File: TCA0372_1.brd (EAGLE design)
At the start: 100 x 80 mm, 30 parts, among them IC1R1 AQY212_1, IC2 Dil16: 4xAQY212, IC4 TCA0372, Q1 BSS101, Q2 BSS101

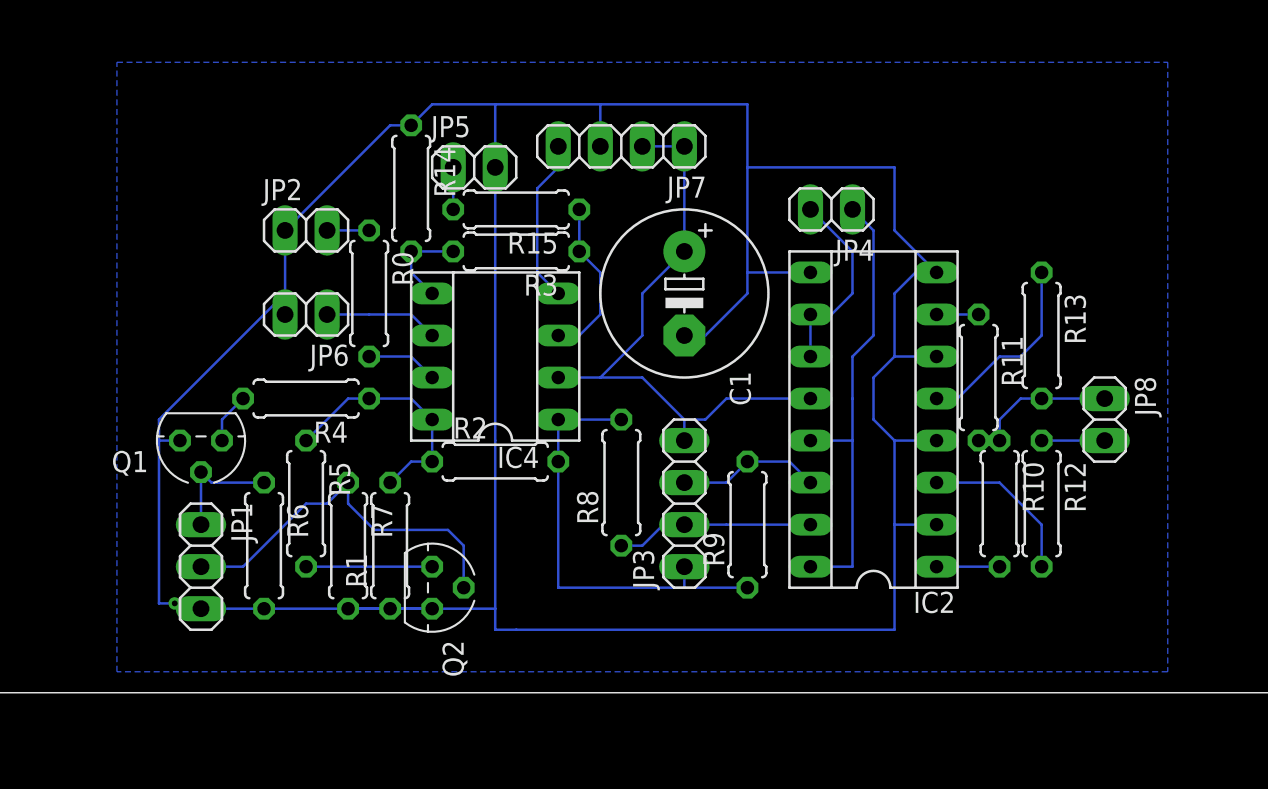
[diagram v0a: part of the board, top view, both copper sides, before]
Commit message: Add files via upload
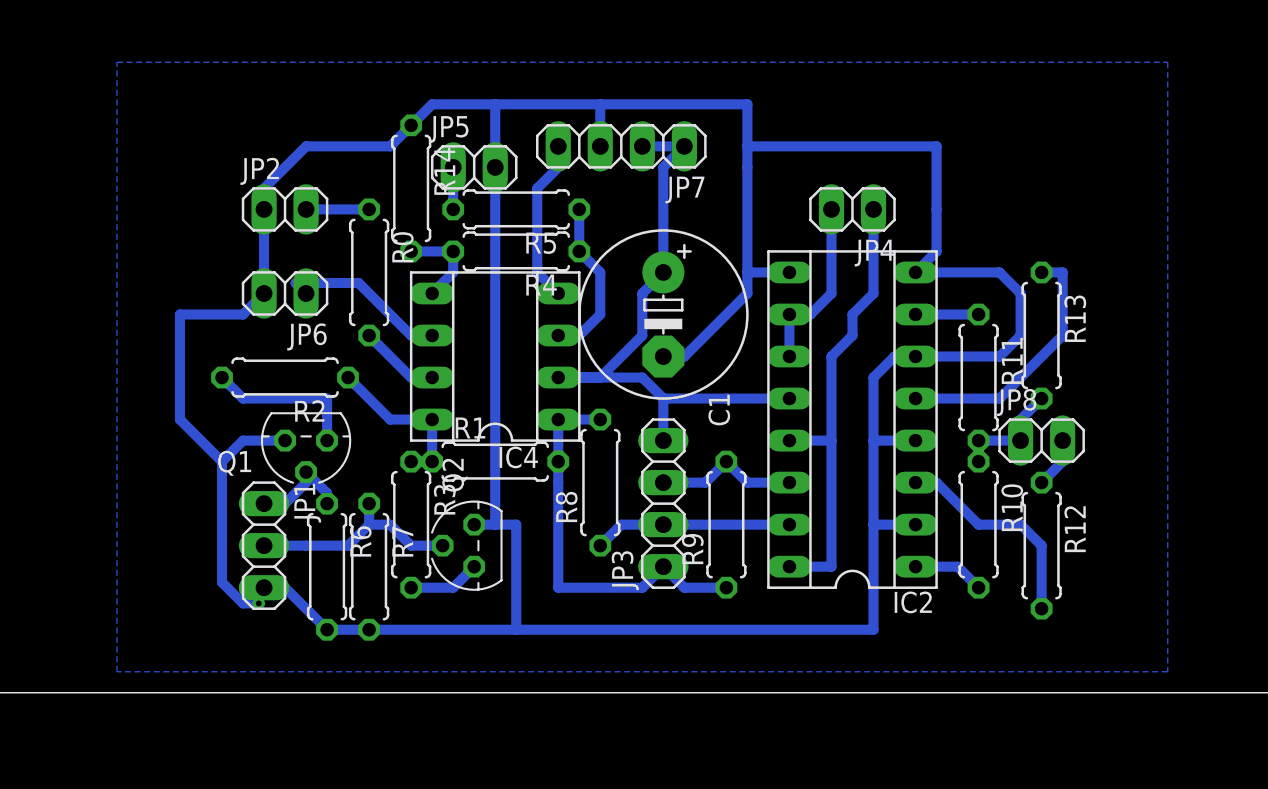
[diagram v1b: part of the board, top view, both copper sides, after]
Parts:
- removed R15: 27k, rcl:0207/7
- R14: value 33k -> 100M
- R3: value 68k -> 6.6k
- R4: value 33.2k -> 0
- R5: value 8.2k -> 0
- moved R5 21.8 mm to (39.4, 29.2), turned to 180 degrees
- moved R3 17.7 mm to (33.0, 10.2), turned to 270 degrees
- moved R4 15.5 mm to (39.4, 26.7)
- moved R2 13.7 mm to (25.4, 19.1), turned to 180 degrees
- moved R1 8.13 mm to (38.1, 14.0), turned to 0 degrees
- moved Q1 6.35 mm to (26.7, 15.2)
- moved JP8 4.02 mm to (71.1, 15.2), turned to 0 degrees
- moved R6 4.02 mm to (27.9, 7.62)
- moved JP1 4.02 mm to (24.1, 8.89)
- moved Q2 3.59 mm to (36.8, 8.89), turned to 90 degrees
- moved R12 2.54 mm to (71.1, 8.89)
- moved C1 1.80 mm to (48.3, 22.9)
- moved JP2 1.80 mm to (25.4, 29.2)
- moved JP6 1.80 mm to (25.4, 24.1)
- moved R7 1.80 mm to (30.5, 7.62)
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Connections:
- removed net N$14: IC4.1, JP3.1, R2.2, R8.2, R9.1
- removed net N$4: IC4.8, R1.2, R2.1, R4.1, R5.1
- new net N$21: IC4.1, JP3.1, R1.2, R8.2, R9.1
- new net N$22: IC4.8, R1.1, R2.1, R3.1
- net GND: no longer R1.1
- net N$1: now also R4.2; no longer R3.2
- net N$13: now also R4.1, R5.1; no longer R15.1, R3.1
- net N$20: now also R5.2; no longer R15.2
- net N$5: now also R2.2; no longer R4.2
- net N$6: now also R3.2; no longer R5.2
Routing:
- net N$14: track 26.7 -> 0.00 mm
- net N$21: track 0.00 -> 23.9 mm
- net N$4: track 14.8 -> 0.00 mm
- net N$22: track 0.00 -> 9.94 mm
- net N$8: track 22.8 -> 13.1 mm
- net N$5: track 3.07 -> 9.42 mm
- net GND: track 218.1 -> 223.5 mm
- net V+: track 36.7 -> 40.7 mm
- net N$15: track 11.7 -> 15.5 mm
- net N$9: track 6.88 -> 10.5 mm
- net N$6: track 7.62 -> 4.34 mm
- net N$10: track 9.94 -> 13.0 mm
- net N$19: track 9.42 -> 6.88 mm
- net N$12: track 2.54 -> 3.81 mm
- net N$18: track 2.54 -> 3.81 mm
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
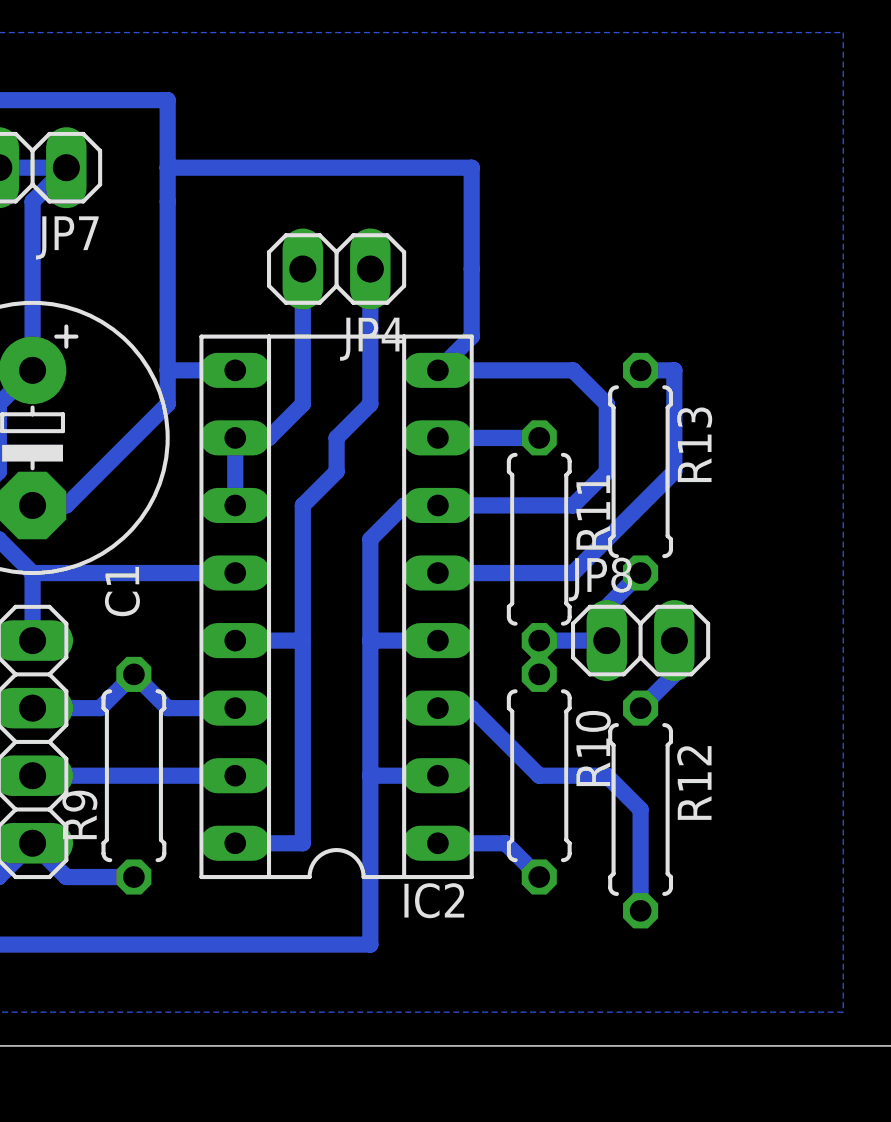
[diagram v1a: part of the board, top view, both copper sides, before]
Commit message: Add files via upload
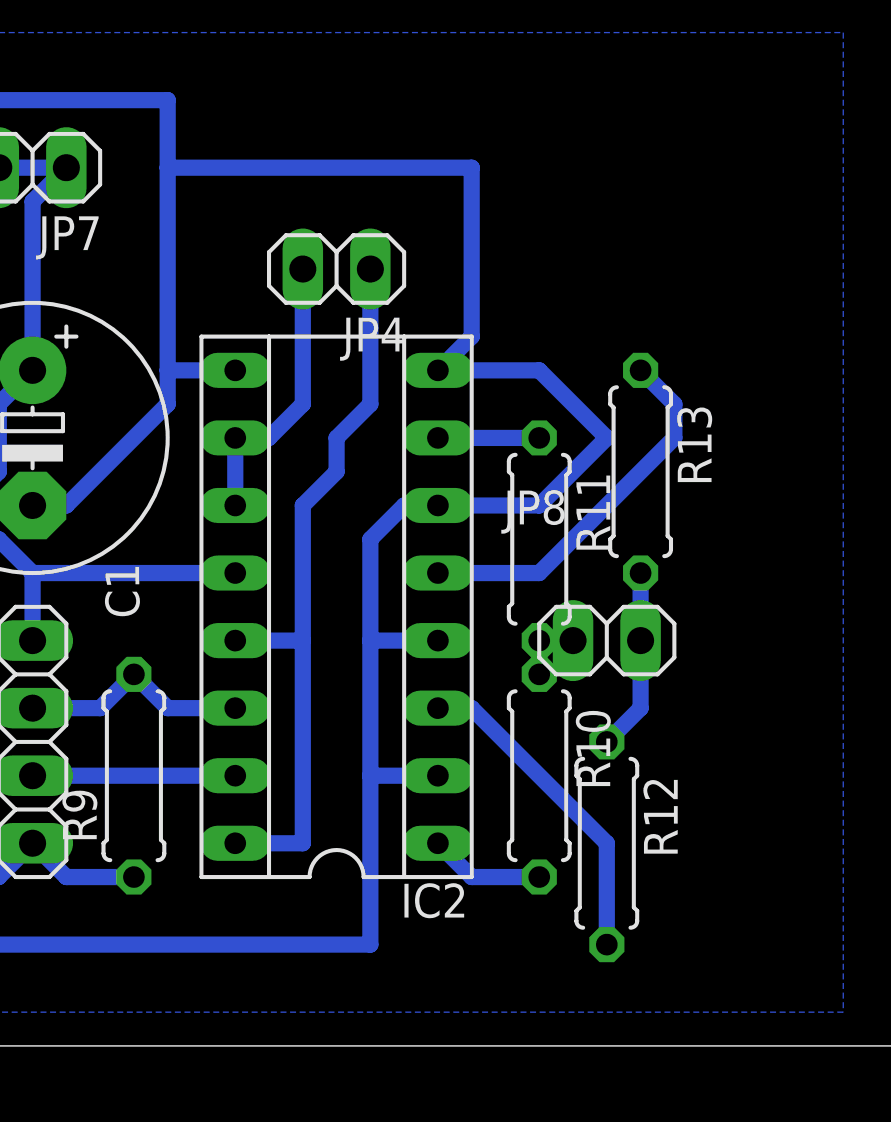
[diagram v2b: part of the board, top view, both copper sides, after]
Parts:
- JP8: value from Pin19/20 -> from Pin19->1/20->2
- moved R12 1.80 mm to (69.8, 7.62)
- moved JP8 1.27 mm to (69.8, 15.2)
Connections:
- net N$16: now also R13.2
- net N$19: no longer R13.2
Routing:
- net N$19: track 6.88 -> 2.54 mm
- net N$16: track 3.07 -> 6.88 mm
- net N$15: track 15.5 -> 14.1 mm
- net GND: track 223.5 -> 222.0 mm
- net N$10: track 13.0 -> 12.3 mm
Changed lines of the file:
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@@
 <attribute name="VALUE" x="62.23" y="32.385" size="1.27" layer="27" rot="R180"/>
 </element>
-<element name="JP8" library="pinhead" library_urn="urn:adsk.eagle:library:325" package="1X02" package3d_urn="urn:adsk.eagle:package:22435/2" value="from Pin19/20" x="71.12" y="15.24" smashed="yes">
-<attribute name="NAME" x="68.5038" y="17.0688" size="1.27" layer="25" ratio="10"/>
-<attribute name="VALUE" x="68.58" y="12.065" size="1.27" layer="27"/>
+<element name="JP8" library="pinhead" library_urn="urn:adsk.eagle:library:325" package="1X02" package3d_urn="urn:adsk.eagle:package:22435/2" value="from Pin19-&gt;1/20-&gt;2" x="69.85" y="15.24" smashed="yes">
+<attribute name="NAME" x="65.9638" y="19.6088" size="1.27" layer="25" ratio="10"/>
+<attribute name="VALUE" x="67.31" y="12.065" size="1.27" layer="27"/>
 </element>
 <element name="JP5" library="pinhead" library_urn="urn:adsk.eagle:library:325" package="1X02" package3d_urn="urn:adsk.eagle:package:22435/2" value="to Base" x="36.83" y="31.75" smashed="yes">
@@
 <attribute name="NAME" x="68.707" y="21.59" size="1.27" layer="25" ratio="10" rot="R270"/>
 <attribute name="SPICEPREFIX" value="R" x="67.31" y="19.05" size="1.778" layer="27" rot="R270" display="off"/>
-<attribute name="VALUE" x="66.7512" y="21.336" size="1.27" layer="27" ratio="10" rot="R270"/>
-</element>
-<element name="R12" library="rcl" library_urn="urn:adsk.eagle:library:334" package="0207/7" package3d_urn="urn:adsk.eagle:package:23493/1" value="470" x="71.12" y="8.89" smashed="yes" rot="R270">
-<attribute name="NAME" x="72.517" y="11.43" size="1.27" layer="25" ratio="10" rot="R270"/>
-<attribute name="SPICEPREFIX" value="R" x="71.12" y="8.89" size="1.778" layer="27" rot="R270" display="off"/>
-<attribute name="VALUE" x="70.5612" y="11.176" size="1.27" layer="27" ratio="10" rot="R270"/>
+<attribute name="VALUE" x="66.7512" y="20.066" size="1.27" layer="27" ratio="10" rot="R270"/>
+</element>
+<element name="R12" library="rcl" library_urn="urn:adsk.eagle:library:334" package="0207/7" package3d_urn="urn:adsk.eagle:package:23493/1" value="470" x="69.85" y="7.62" smashed="yes" rot="R270">
+<attribute name="NAME" x="71.247" y="10.16" size="1.27" layer="25" ratio="10" rot="R270"/>
+<attribute name="SPICEPREFIX" value="R" x="69.85" y="7.62" size="1.778" layer="27" rot="R270" display="off"/>
+<attribute name="VALUE" x="70.5612" y="9.906" size="1.27" layer="27" ratio="10" rot="R270"/>
 </element>
 <element name="R13" library="rcl" library_urn="urn:adsk.eagle:library:334" package="0207/7" package3d_urn="urn:adsk.eagle:package:23493/1" value="470" x="71.12" y="21.59" smashed="yes" rot="R270">
@@
 <wire x1="44.45" y1="35.56" x2="53.34" y2="35.56" width="0.6096" layer="16"/>
 <wire x1="53.34" y1="35.56" x2="53.34" y2="33.02" width="0.6096" layer="16"/>
-<wire x1="53.34" y1="31.75" x2="53.34" y2="25.4" width="0.6096" layer="16"/>
+<wire x1="53.34" y1="33.02" x2="53.34" y2="25.4" width="0.6096" layer="16"/>
 <wire x1="53.34" y1="25.4" x2="55.88" y2="25.4" width="0.6096" layer="16"/>
 <wire x1="48.26" y1="20.32" x2="49.53" y2="20.32" width="0.6096" layer="16"/>
@@
 <wire x1="36.83" y1="10.16" x2="38.1" y2="10.16" width="0.6096" layer="16"/>
 <wire x1="53.34" y1="33.02" x2="64.77" y2="33.02" width="0.6096" layer="16"/>
-<wire x1="64.77" y1="33.02" x2="64.77" y2="29.21" width="0.6096" layer="16"/>
-<wire x1="64.77" y1="29.21" x2="64.77" y2="26.67" width="0.6096" layer="16"/>
+<wire x1="64.77" y1="33.02" x2="64.77" y2="26.67" width="0.6096" layer="16"/>
 <wire x1="63.5" y1="20.32" x2="62.23" y2="20.32" width="0.6096" layer="16"/>
 <wire x1="62.23" y1="20.32" x2="60.96" y2="19.05" width="0.6096" layer="16"/>
@@
 <wire x1="60.96" y1="10.16" x2="63.5" y2="10.16" width="0.6096" layer="16"/>
 <wire x1="60.96" y1="15.24" x2="63.5" y2="15.24" width="0.6096" layer="16"/>
-<wire x1="68.58" y1="20.32" x2="63.5" y2="20.32" width="0.6096" layer="16"/>
-<wire x1="63.5" y1="25.4" x2="68.58" y2="25.4" width="0.6096" layer="16"/>
-<wire x1="68.58" y1="25.4" x2="69.85" y2="24.13" width="0.6096" layer="16"/>
-<wire x1="69.85" y1="24.13" x2="69.85" y2="21.59" width="0.6096" layer="16"/>
-<wire x1="69.85" y1="21.59" x2="68.58" y2="20.32" width="0.6096" layer="16"/>
 <wire x1="64.77" y1="26.67" x2="63.5" y2="25.4" width="0.6096" layer="16"/>
-<wire x1="53.34" y1="33.02" x2="53.34" y2="31.75" width="0.6096" layer="16"/>
+<wire x1="67.31" y1="25.4" x2="69.85" y2="22.86" width="0.6096" layer="16"/>
+<wire x1="63.5" y1="25.4" x2="67.31" y2="25.4" width="0.6096" layer="16"/>
+<wire x1="69.85" y1="22.86" x2="67.31" y2="20.32" width="0.6096" layer="16"/>
+<wire x1="67.31" y1="20.32" x2="63.5" y2="20.32" width="0.6096" layer="16"/>
 </signal>
 <signal name="N$7">
@@
 <contactref element="R10" pad="2"/>
 <contactref element="IC2" pad="1"/>
-<wire x1="63.5" y1="7.62" x2="66.04" y2="7.62" width="0.6096" layer="16"/>
-<wire x1="66.04" y1="7.62" x2="67.31" y2="6.35" width="0.6096" layer="16"/>
+<wire x1="67.31" y1="6.35" x2="64.77" y2="6.35" width="0.6096" layer="16"/>
+<wire x1="63.5" y1="7.62" x2="64.77" y2="6.35" width="0.6096" layer="16"/>
 </signal>
 <signal name="N$18">
 <contactref element="R11" pad="1"/>
 <contactref element="IC2" pad="7"/>
-<wire x1="63.5" y1="22.86" x2="67.31" y2="22.86" width="0.6096" layer="16"/>
+<wire x1="67.31" y1="22.86" x2="63.5" y2="22.86" width="0.6096" layer="16"/>
 </signal>
 <signal name="N$19">
@@
 <contactref element="JP8" pad="1"/>
 <contactref element="R11" pad="2"/>
-<contactref element="R13" pad="2"/>
 <wire x1="67.31" y1="15.24" x2="67.31" y2="13.97" width="0.6096" layer="16"/>
-<wire x1="67.31" y1="15.24" x2="69.85" y2="15.24" width="0.6096" layer="16"/>
-<wire x1="69.85" y1="16.51" x2="69.85" y2="15.24" width="0.6096" layer="16"/>
-<wire x1="71.12" y1="17.78" x2="69.85" y2="16.51" width="0.6096" layer="16"/>
+<wire x1="67.31" y1="15.24" x2="68.58" y2="15.24" width="0.6096" layer="16"/>
 </signal>
 <signal name="N$1">
@@
 <contactref element="JP8" pad="2"/>
 <contactref element="R12" pad="1"/>
-<wire x1="71.12" y1="12.7" x2="72.39" y2="13.97" width="0.6096" layer="16"/>
-<wire x1="72.39" y1="13.97" x2="72.39" y2="15.24" width="0.6096" layer="16"/>
+<wire x1="71.12" y1="12.7" x2="71.12" y2="15.24" width="0.6096" layer="16"/>
+<wire x1="71.12" y1="12.7" x2="69.85" y2="11.43" width="0.6096" layer="16"/>
+<contactref element="R13" pad="2"/>
+<wire x1="71.12" y1="17.78" x2="71.12" y2="15.24" width="0.6096" layer="16"/>
 </signal>
 <signal name="N$23">
@@
 <contactref element="R12" pad="2"/>
 <wire x1="63.5" y1="12.7" x2="64.77" y2="12.7" width="0.6096" layer="16"/>
-<wire x1="64.77" y1="12.7" x2="67.31" y2="10.16" width="0.6096" layer="16"/>
-<wire x1="67.31" y1="10.16" x2="69.85" y2="10.16" width="0.6096" layer="16"/>
-<wire x1="69.85" y1="10.16" x2="71.12" y2="8.89" width="0.6096" layer="16"/>
-<wire x1="71.12" y1="8.89" x2="71.12" y2="5.08" width="0.6096" layer="16"/>
+<wire x1="64.77" y1="12.7" x2="69.85" y2="7.62" width="0.6096" layer="16"/>
+<wire x1="69.85" y1="7.62" x2="69.85" y2="3.81" width="0.6096" layer="16"/>
 </signal>
 <signal name="N$15">
 <contactref element="IC2" pad="5"/>
 <contactref element="R13" pad="1"/>
-<wire x1="63.5" y1="17.78" x2="68.58" y2="17.78" width="0.6096" layer="16"/>
-<wire x1="68.58" y1="17.78" x2="72.39" y2="21.59" width="0.6096" layer="16"/>
-<wire x1="72.39" y1="21.59" x2="72.39" y2="25.4" width="0.6096" layer="16"/>
-<wire x1="72.39" y1="25.4" x2="71.12" y2="25.4" width="0.6096" layer="16"/>
+<wire x1="63.5" y1="17.78" x2="67.31" y2="17.78" width="0.6096" layer="16"/>
+<wire x1="71.12" y1="25.4" x2="72.39" y2="24.13" width="0.6096" layer="16"/>
+<wire x1="72.39" y1="24.13" x2="72.39" y2="22.86" width="0.6096" layer="16"/>
+<wire x1="72.39" y1="22.86" x2="67.31" y2="17.78" width="0.6096" layer="16"/>
 </signal>
 <signal name="N$21">
